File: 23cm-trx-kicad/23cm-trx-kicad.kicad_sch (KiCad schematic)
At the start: 37 parts, among them J2 LCD I2C, SW1 RotaryEncoder_Switch, U2 L78L09_SOT89, U3 LM741, U4 LM386

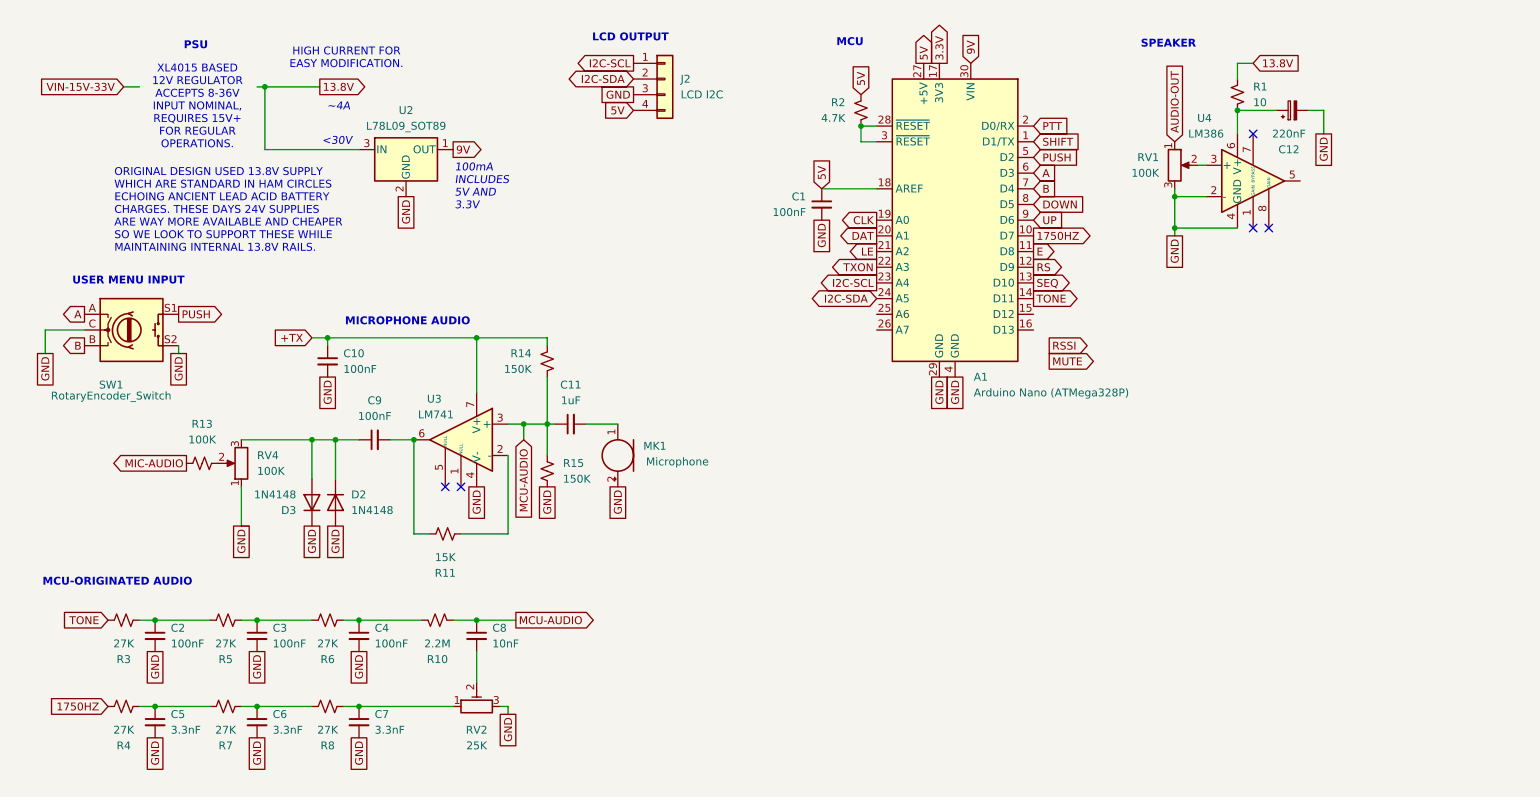
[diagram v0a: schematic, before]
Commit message: Further schematic work
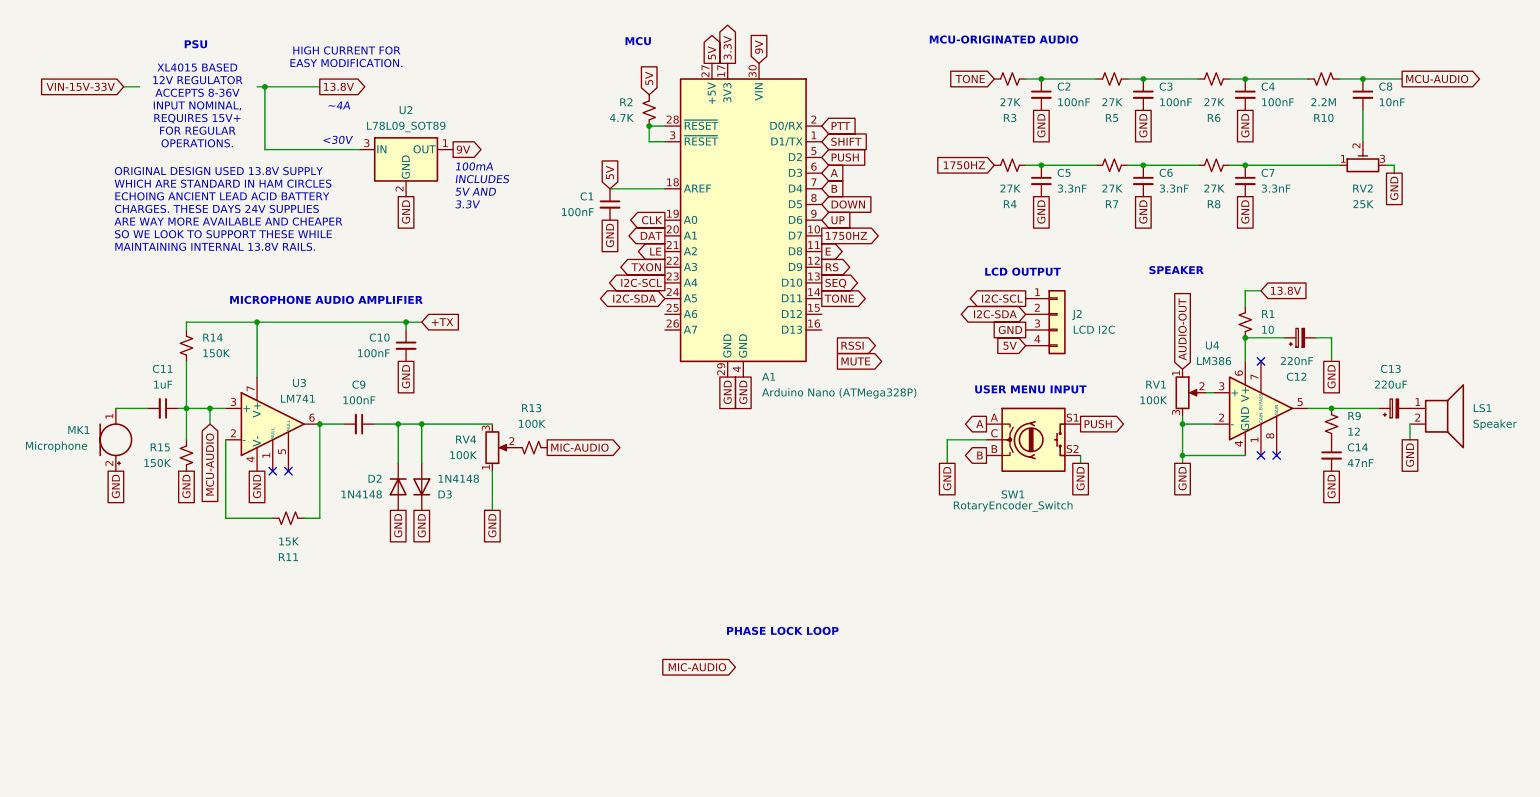
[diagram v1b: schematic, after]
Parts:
- added C13: 220uF, symbol Device:C_Polarized_Small
- added C14: 47nF, symbol Device:C_Small
- added LS1: Speaker, symbol Device:Speaker
- added R9: 12, symbol Device:R_Small_US
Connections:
- net GND: now also C14.2, LS1.2
- net at U4.5: now also C13.1, R9.1
- new net: C13.2, LS1.1
- new net: C14.1, R9.2
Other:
- note added: "MICROPHONE AUDIO AMPLIFIER"
- note added: "PHASE LOCK LOOP"
- note removed: "MICROPHONE AUDIO"
- moved on the sheet: A1, C1, C10, C11, C12, C2, C3, C4, C5, C6, C7, C8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
